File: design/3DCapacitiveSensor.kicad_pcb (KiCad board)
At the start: 2 copper layers, 14 parts, among them J1 Pin Socket, J2 X_shield, J3 Y_shield, J4 X_plate, J5 Y_plate, J6 Z_plate, J7 3V, J8 Z_shield

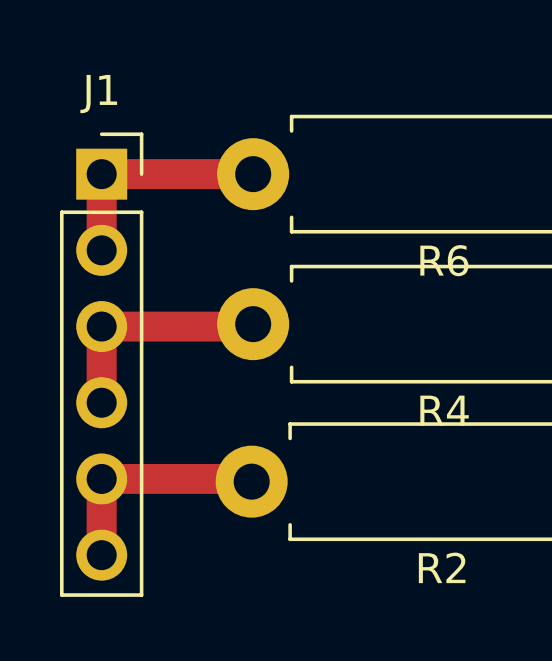
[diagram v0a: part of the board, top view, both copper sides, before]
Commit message: Update schematic
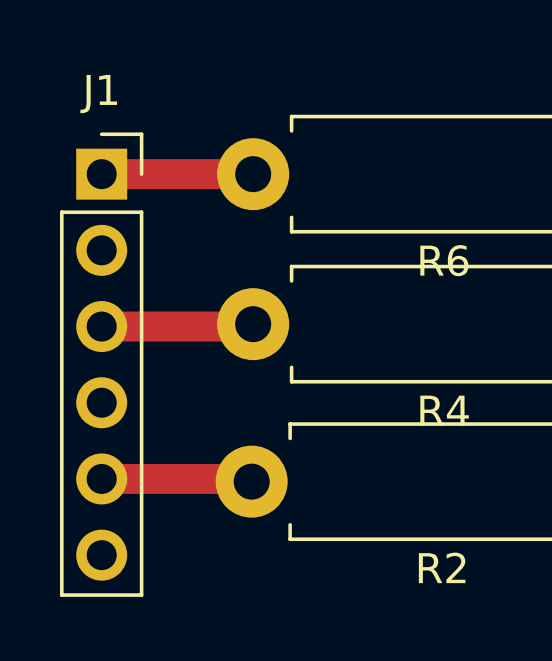
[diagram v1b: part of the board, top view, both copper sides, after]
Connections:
- J1 pad 1: /X_ADC -> /X_pin
- J1 pad 2: /X_ADC -> (no net)
- J1 pad 3: /Y_ADC -> /Y_pin
- J1 pad 4: /Y_ADC -> (no net)
- J1 pad 5: /Z_ADC -> /Z_pin
- J1 pad 6: /Z_ADC -> (no net)
- R2 pad 2: /Z_ADC -> /Z_pin
- R4 pad 2: /Y_ADC -> /Y_pin
- R6 pad 2: /X_ADC -> /X_pin
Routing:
- net /Y_ADC: track 7.62 -> 0.00 mm
- net /X_ADC: track 7.59 -> 0.00 mm
- net /Z_ADC: track 7.58 -> 0.00 mm
- net /Y_pin: track 0.00 -> 5.08 mm
- net /X_pin: track 0.00 -> 5.05 mm
- net /Z_pin: track 0.00 -> 5.04 mm
